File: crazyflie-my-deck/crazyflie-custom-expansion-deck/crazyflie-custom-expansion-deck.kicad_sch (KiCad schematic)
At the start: 16 parts, among them J1 Conn_01x10, J2 Conn_01x06_Male, J3 Conn_01x10

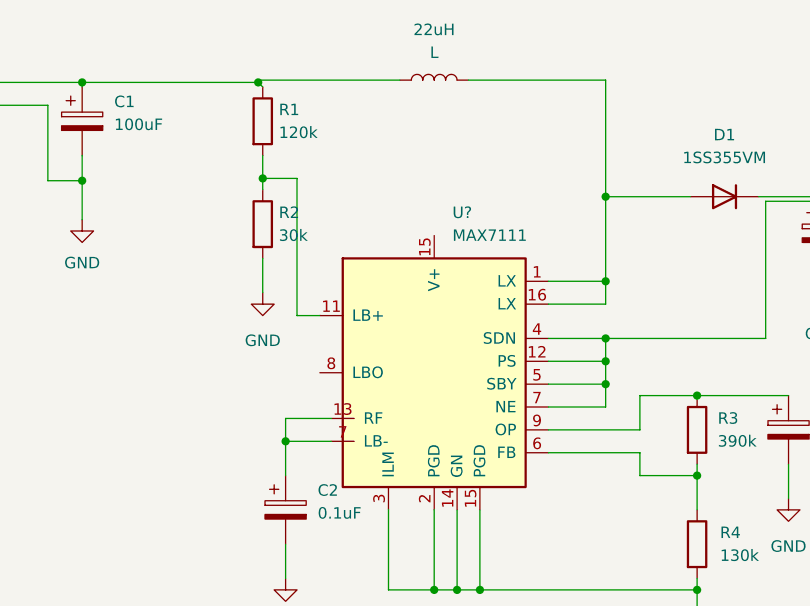
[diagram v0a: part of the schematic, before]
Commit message: Fixes
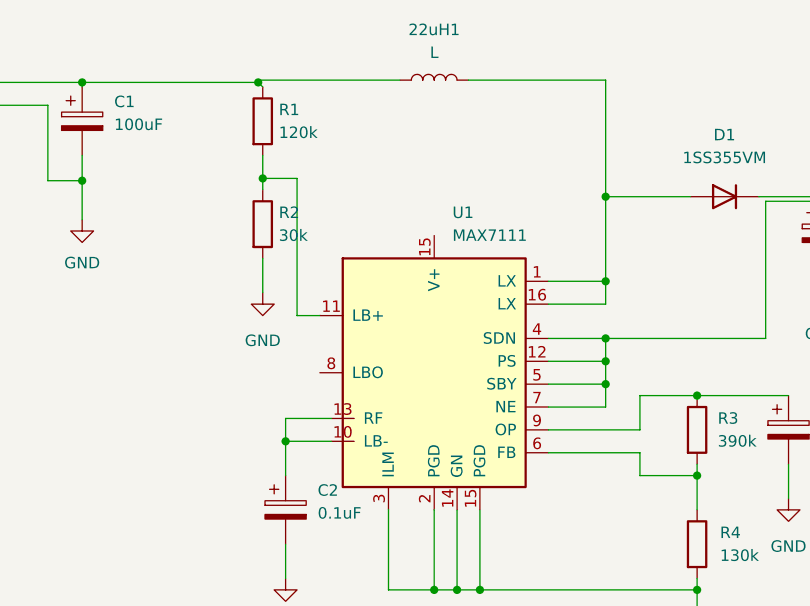
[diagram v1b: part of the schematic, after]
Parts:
- removed U?: MAX7111, Package_SO:SOIC-16_3.9x9.9mm_P1.27mm, symbol Battery_Management:MAX7111
- added U1: MAX7111, Package_SO:SOIC-16_3.9x9.9mm_P1.27mm, symbol Battery_Management:MAX7111
- renumbered 22uH to 22uH1
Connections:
- net GND: now also U1.14 (GN), U1.15 (V+), U1.2 (PGD), U1.3 (ILM)
- net at C3.1, R3.1: now also U1.9 (OP)
- net at R3.2, R4.1: now also U1.6 (FB)
- net at 22uH1.2, D1.2 (A): now also U1.1 (LX), U1.16 (LX)
- net at R1.2, R2.1: now also U1.11 (LB+)
- net at C4.1, D1.1 (K): now also U1.12 (PS), U1.4 (SDN), U1.5 (SBY), U1.7 (NE)
- net at C2.1: now also U1.10 (LB-), U1.13 (RF)
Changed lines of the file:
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@@
     (pin "1")
+  )
+  (symbol (lib_id "Battery_Management:MAX7111") (at 90.17 97.79 0) (unit 1)
+    (in_bom yes) (on_board yes) (fields_autoplaced)
+    (property "Reference" "U1" (id 0) (at 92.1894 80.01 0)
+      (effects (font (size 1.27 1.27)) (justify left))
+    )
+    (property "Value" "MAX7111" (id 1) (at 92.1894 82.55 0)
+      (effects (font (size 1.27 1.27)) (justify left))
+    )
+    (property "Footprint" "Package_SO:SOIC-16_3.9x9.9mm_P1.27mm" (id 2) (at 90.17 115.57 0)
+      (effects (font (size 1.27 1.27)) hide)
+    )
+    (property "Datasheet" "https://datasheets.maximintegrated.com/en/ds/MAX712-MAX713.pdf" (id 3) (at 72.39 80.01 0)
+      (effects (font (size 1.27 1.27)) hide)
+    )
+    (pin "1")
+    (pin "11")
+    (pin "12")
+    (pin "13")
+    (pin "14")
+    (pin "15")
+    (pin "15")
+    (pin "16")
+    (pin "2")
+    (pin "3")
+    (pin "4")
+    (pin "5")
+    (pin "6")
+    (pin "10")
+    (pin "7")
+    (pin "8")
+    (pin "9")
   )
   (symbol (lib_id "Connector_Generic:Conn_01x10") (at 188.214 114.808 0) (unit 1)
@@
   (symbol (lib_id "Device:L") (at 90.17 65.278 90) (unit 1)
     (in_bom yes) (on_board yes) (fields_autoplaced)
-    (property "Reference" "22uH" (id 0) (at 90.17 59.69 90))
+    (property "Reference" "22uH1" (id 0) (at 90.17 59.69 90))
     (property "Value" "L" (id 1) (at 90.17 62.23 90))
     (property "Footprint" "Inductor_SMD:L_1210_3225Metric" (id 2) (at 90.17 65.278 0)
@@
     )
     (pin "1")
-  )
-  (symbol (lib_id "Battery_Management:MAX7111") (at 90.17 97.79 0) (unit 1)
-    (in_bom yes) (on_board yes) (fields_autoplaced)
-    (property "Reference" "U?" (id 0) (at 92.1894 80.01 0)
-      (effects (font (size 1.27 1.27)) (justify left))
-    )
-    (property "Value" "MAX7111" (id 1) (at 92.1894 82.55 0)
-      (effects (font (size 1.27 1.27)) (justify left))
-    )
-    (property "Footprint" "Package_SO:SOIC-16_3.9x9.9mm_P1.27mm" (id 2) (at 90.17 115.57 0)
-      (effects (font (size 1.27 1.27)) hide)
-    )
-    (property "Datasheet" "https://datasheets.maximintegrated.com/en/ds/MAX712-MAX713.pdf" (id 3) (at 72.39 80.01 0)
-      (effects (font (size 1.27 1.27)) hide)
-    )
-    (pin "1")
-    (pin "11")
-    (pin "12")
-    (pin "13")
-    (pin "14")
-    (pin "15")
-    (pin "15")
-    (pin "16")
-    (pin "2")
-    (pin "3")
-    (pin "4")
-    (pin "5")
-    (pin "6")
-    (pin "7")
-    (pin "7")
-    (pin "9")
-    (pin "8")
   )
   (symbol (lib_id "Diode:1SS355VM") (at 122.428 78.232 0) (mirror y) (unit 1)
@@
     )
     (path "/63f68aae-215d-48f8-934a-2726f16762b6"
-      (reference "22uH") (unit 1) (value "L") (footprint "Inductor_SMD:L_1210_3225Metric")
+      (reference "22uH1") (unit 1) (value "L") (footprint "Inductor_SMD:L_1210_3225Metric")
     )
     (path "/4d3e9d1d-ce51-42ca-be59-2c77834705f0"
@@
       (reference "R4") (unit 1) (value "130k") (footprint "Resistor_SMD:R_0805_2012Metric")
     )
-    (path "/a28b1465-c59f-4464-af17-db4f1321b7fc"
-      (reference "U?") (unit 1) (value "MAX7111") (footprint "Package_SO:SOIC-16_3.9x9.9mm_P1.27mm")
-    )
-  )
+    (path "/32370ee8-91f4-40c5-9f1f-b1b5884d4ee2"
+      (reference "U1") (unit 1) (value "MAX7111") (footprint "Package_SO:SOIC-16_3.9x9.9mm_P1.27mm")
+    )
+  )
